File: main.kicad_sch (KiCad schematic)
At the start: 0 parts

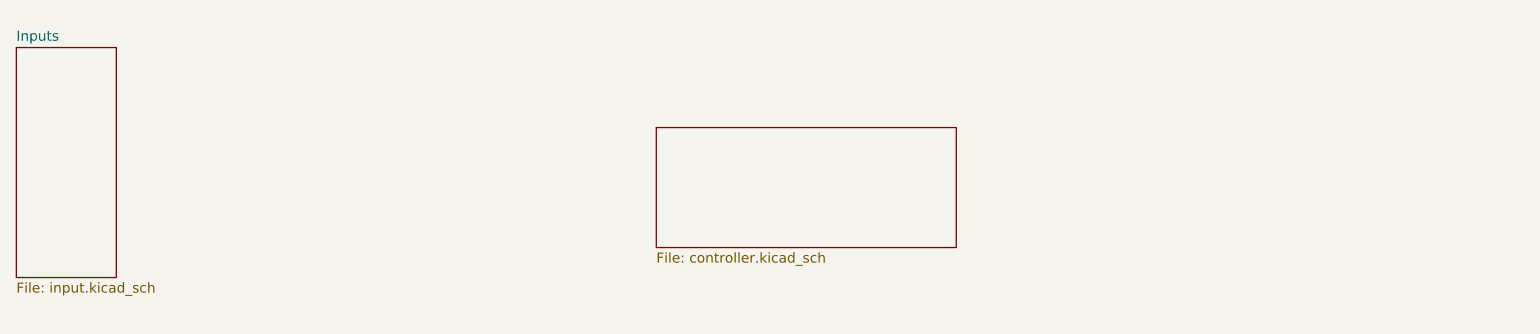
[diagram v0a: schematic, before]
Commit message: post solar meeting with ezzat
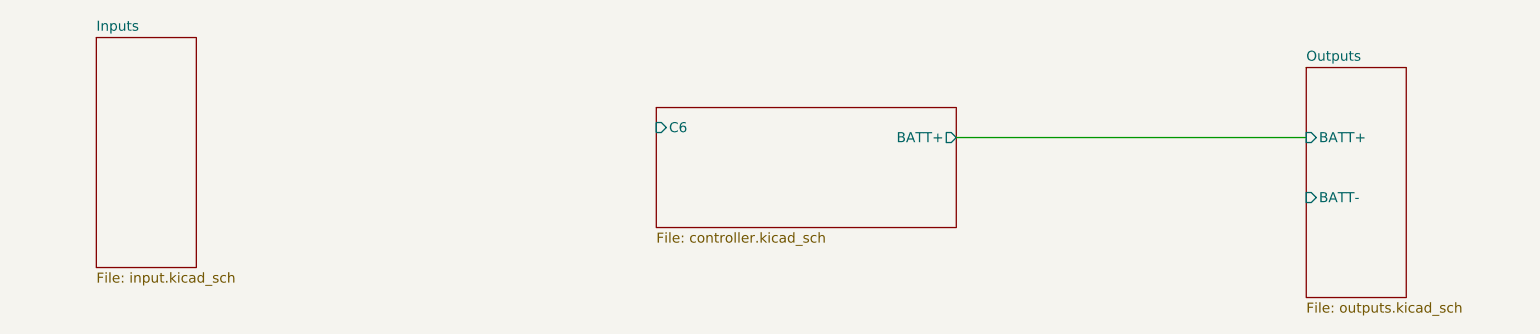
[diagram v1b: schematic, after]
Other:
- added sheet Outputs (outputs.kicad_sch)
- sheet BMS ports: added BATT+, C6; removed none
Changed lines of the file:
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@@
 	(generator_version "9.0")
 	(paper "A4")
+	(wire
+		(pts
+			(xy 158.75 91.44) (xy 203.2 91.44)
+		)
+		(stroke
+			(width 0)
+			(type default)
+		)
+	)
 	(sheet
-		(at 39.37 80.01)
+		(at 203.2 82.55)
+		(size 12.7 29.21)
+		(exclude_from_sim no)
+		(in_bom yes)
+		(on_board yes)
+		(dnp no)
+		(fields_autoplaced yes)
+		(stroke
+			(width 0.1524)
+			(type solid)
+		)
+		(fill
+			(color 0 0 0 0.0000)
+		)
+		(property "Sheetname" "Outputs"
+			(at 203.2 81.8384 0)
+			(effects
+				(font
+					(size 1.27 1.27)
+				)
+				(justify left bottom)
+			)
+		)
+		(property "Sheetfile" "outputs.kicad_sch"
+			(at 203.2 112.3446 0)
+			(effects
+				(font
+					(size 1.27 1.27)
+				)
+				(justify left top)
+			)
+		)
+		(pin "BATT+" input
+			(at 203.2 91.44 180)
+			(effects
+				(font
+					(size 1.27 1.27)
+				)
+				(justify left)
+			)
+		)
+		(pin "BATT-" input
+			(at 203.2 99.06 180)
+			(effects
+				(font
+					(size 1.27 1.27)
+				)
+				(justify left)
+			)
+		)
+		(instances
+			(project "BMS"
+				(path "/124184ba-5d68-4d9f-8da6-acc6720ab30b/93f9b420-7cce-46a9-9201-666f07a18f85"
+					(page "2")
+				)
+			)
+		)
+	)
+	(sheet
+		(at 49.53 78.74)
 		(size 12.7 29.21)
 		(exclude_from_sim no)
@@
 		)
 		(property "Sheetname" "Inputs"
-			(at 39.37 79.2984 0)
+			(at 49.53 78.0284 0)
 			(effects
 				(font
@@
 		)
 		(property "Sheetfile" "input.kicad_sch"
-			(at 39.37 109.8046 0)
+			(at 49.53 108.5346 0)
 			(effects
 				(font
@@
 			)
 		)
-		(instances
-			(project "BMS"
-				(path "/124184ba-5d68-4d9f-8da6-acc6720ab30b/9364b786-ab76-48f0-917a-74b98e30a261"
-					(page "7")
-				)
-			)
-		)
 	)
 	(sheet
-		(at 120.65 90.17)
+		(at 120.65 87.63)
 		(size 38.1 15.24)
 		(exclude_from_sim no)
@@
 		)
 		(property "Sheetname" "BMS"
-			(at 120.65 89.4584 0)
+			(at 120.65 86.9184 0)
 			(effects
 				(font
@@
 		)
 		(property "Sheetfile" "controller.kicad_sch"
-			(at 120.65 105.9946 0)
+			(at 120.65 103.4546 0)
 			(effects
 				(font
@@
 			)
 		)
-		(instances
-			(project "BMS"
-				(path "/124184ba-5d68-4d9f-8da6-acc6720ab30b/9364b786-ab76-48f0-917a-74b98e30a261"
-					(page "5")
+		(pin "BATT+" output
+			(at 158.75 91.44 0)
+			(effects
+				(font
+					(size 1.27 1.27)
 				)
+				(justify right)
 			)
 		)
+		(pin "C6" input
+			(at 120.65 90.17 180)
+			(effects
+				(font
+					(size 1.27 1.27)
+				)
+				(justify left)
+			)
+		)
